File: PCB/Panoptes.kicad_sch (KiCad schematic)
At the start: 104 parts, among them J1 Conn_02x05_Odd_Even, J2 Conn_02x10_Odd_Even, J3 Conn_01x02, J4 Conn_01x03, J5 Conn_01x03, J6 Conn_01x02, J7 Conn_01x02, Q1 MMBT3904, U1 SE555D, U2 ADS7882, U3 L79L05_SOT89, U4 L78L33_SOT89, U5 L78L05_SOT89, U6 OPA2350UA, U7 OPA2350UA, U8 SK0530

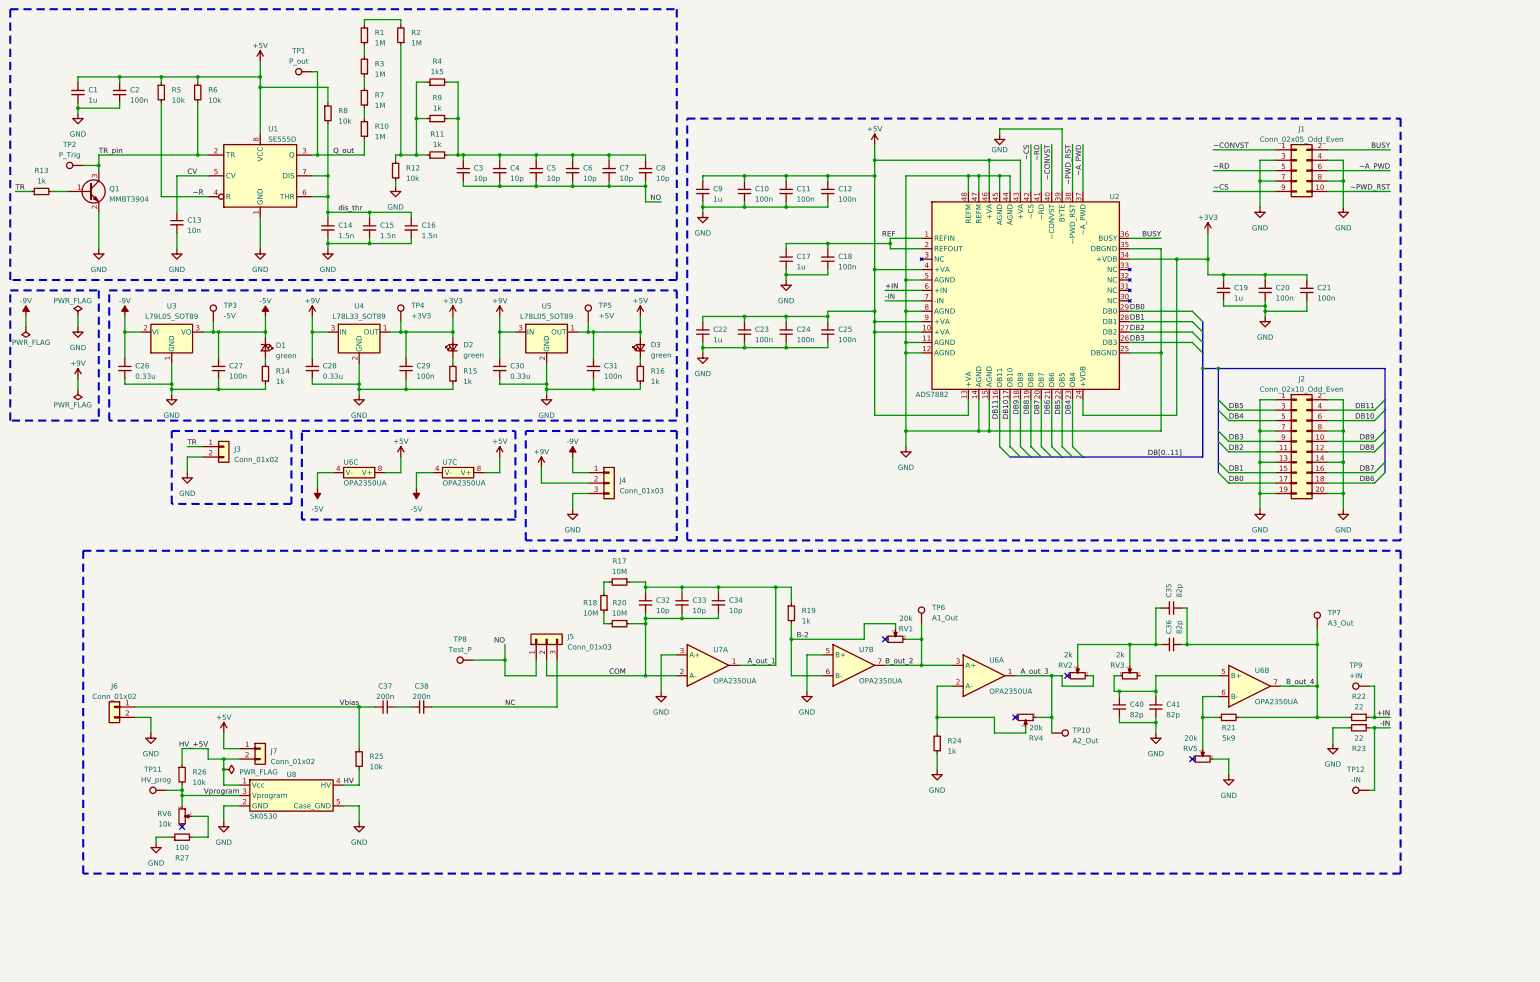
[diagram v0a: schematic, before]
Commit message: V3 completed
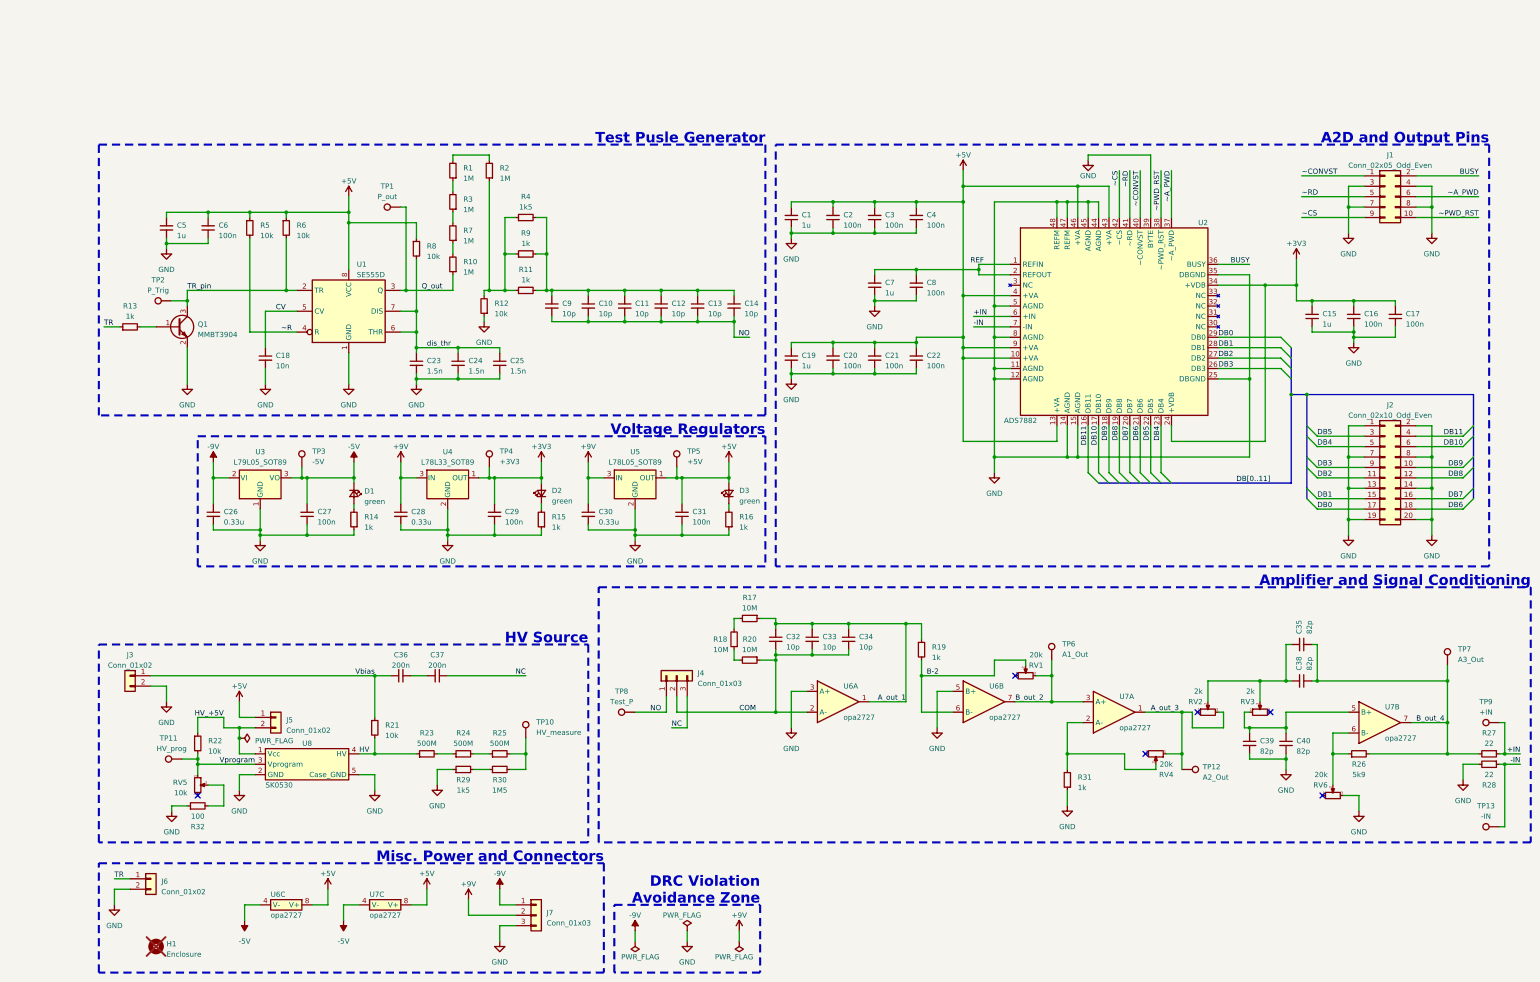
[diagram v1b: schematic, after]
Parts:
- removed U6, U7: OPA2350UA, Package_SO:SOIC-8_3.9x4.9mm_P1.27mm, symbol Panoptes:OPA2350UA
- added H1: Enclosure, n/a, symbol Mechanical:MountingHole
- added R23, R24, R25: 500M, Resistor_THT:R_Axial_DIN0207_L6.3mm_D2.5mm_P7.62mm_Horizontal, symbol Device:R_Small
- added R29: 1k5, Resistor_SMD:R_1206_3216Metric, symbol Device:R_Small
- added R30: 1M5, Resistor_SMD:R_1206_3216Metric, symbol Device:R_Small
- added TP10: HV_measure, TestPoint:TestPoint_Pad_D1.0mm, symbol Connector:TestPoint
- added U6, U7: opa2727, Package_DFN_QFN:DFN-8-1EP_3x3mm_P0.65mm_EP1.55x2.4mm, symbol Panoptes:opa2727
- J1: DK_Detail_Page (none) -> https://www.digikey.com/en/products/detail/sullins-connecto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; DK_PN (none) -> S9202-ND; MPN (none) -> SFH11-PBPC-D05-RA-BK; Manufacturer (none) -> Sullins Connector Solutions
- J2: DK_Detail_Page (none) -> https://www.digikey.com/en/products/detail/sullins-connecto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; DK_PN (none) -> S9205-ND; MPN (none) -> SFH11-PBPC-D10-RA-BK; Manufacturer (none) -> Sullins Connector Solutions
- J4: renamed from J5; DK_Detail_Page (none) -> n/a; DK_PN (none) -> n/a; MPN (none) -> n/a; Manufacturer (none) -> n/a
- J5: renamed from J7; DK_Detail_Page (none) -> n/a; DK_PN (none) -> n/a; MPN (none) -> n/a; Manufacturer (none) -> n/a
- J6: renamed from J3; DK_Detail_Page (none) -> https://www.digikey.com/en/products/detail/sullins-connecto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; DK_PN (none) -> S5438-ND; MPN (none) -> PPTC021LGBN-RC; Manufacturer (none) -> Sullins Connector Solutions
- R1, R10, R2, R3, R7: DK_Detail_Page https://www.digikey.com/en/products/detail/stackpole-electronics-inc/RNCF1206BKE1M00/2027096 -> https://www.digikey.com/en/products/detail/stackpole-electronics-inc/RMCF1206FT1M00/1759703; DK_PN RNCF1206BKE1M00CT-ND -> RMCF1206FT1M00CT-ND; MPN RNCF1206BKE1M00 -> RMCF1206FT1M00
- R11, R13, R14, R15, R16, R19, R9: DK_Detail_Page https://www.digikey.com/en/products/detail/stackpole-electronics-inc/RNCS1206BKE1K00/1800333 -> https://www.digikey.com/en/products/detail/stackpole-electronics-inc/RMCF1206FT1K00/1759616; DK_PN RNCS1206BKE1K00CT-ND -> RMCF1206FT1K00CT-ND; MPN RNCS1206BKE1K00 -> RMCF1206FT1K00
- R12, R5, R6, R8: DK_Detail_Page https://www.digikey.com/en/products/detail/stackpole-electronichttps://www.digikey.com/en/products/detail/stackpole-electronics-inc/RNCS1206BKE10K0/1800330s-inc/RNCS1206BKE10K0/1800330 -> https://www.digikey.com/en/products/detail/stackpole-electronics-inc/RMCF1206FT10K0/1759669; DK_PN RNCS1206BKE10K0CT-ND -> RMCF1206FT10K0CT-ND; MPN RNCS1206BKE10K0 -> RMCF1206FT10K0
- R17, R18, R20: DK_Detail_Page https://www.digikey.com/en/products/detail/vishay-beyschlag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 -> https://www.digikey.com/en/products/detail/stackpole-electr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; DK_PN 749-MCA1206MD1005BP500CT-ND -> RMCF1206FT10M0CT-ND; MPN MCA1206MD1005BP500 -> RMCF1206FT10M0; Manufacturer Vishay Dale -> Stackpole Electronics Inc
- R21: renamed from R25; DK_Detail_Page https://www.digikey.com/en/products/detail/stackpole-electronichttps://www.digikey.com/en/products/detail/stackpole-electronics-inc/RNCS1206BKE10K0/1800330s-inc/RNCS1206BKE10K0/1800330 -> https://www.digikey.com/en/products/detail/stackpole-electronics-inc/RMCF1206FT10K0/1759669; DK_PN RNCS1206BKE10K0CT-ND -> RMCF1206FT10K0CT-ND; MPN RNCS1206BKE10K0 -> RMCF1206FT10K0
- R22: renamed from R26; DK_Detail_Page https://www.digikey.com/en/products/detail/stackpole-electronichttps://www.digikey.com/en/products/detail/stackpole-electronics-inc/RNCS1206BKE10K0/1800330s-inc/RNCS1206BKE10K0/1800330 -> https://www.digikey.com/en/products/detail/stackpole-electronics-inc/RMCF1206FT10K0/1759669; DK_PN RNCS1206BKE10K0CT-ND -> RMCF1206FT10K0CT-ND; MPN RNCS1206BKE10K0 -> RMCF1206FT10K0
- R26: renamed from R21; DK_Detail_Page https://www.digikey.com/en/products/detail/panasonic-electr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 -> https://www.digikey.com/en/products/detail/vishay-dale/CRCW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; DK_PN P5.9KBCCT-ND -> 541-5.90KFCT-ND; MPN ERA-8AEB5901V -> CRCW12065K90FKEA; Manufacturer Panasonic Electronic Components -> Vishay Dale
- R27: renamed from R22; DK_Detail_Page https://www.digikey.com/en/products/detail/stackpole-electronics-inc/RTAN1206BKE22R0/6602201 -> https://www.digikey.com/en/products/detail/stackpole-electronics-inc/RMCF1206FT22R0/1759698; DK_PN RTAN1206BKE22R0CT-ND -> RMCF1206FT22R0CT-ND; MPN RTAN1206BKE22R0 -> RMCF1206FT22R0
- R28: renamed from R23; DK_Detail_Page https://www.digikey.com/en/products/detail/stackpole-electronics-inc/RTAN1206BKE22R0/6602201 -> https://www.digikey.com/en/products/detail/stackpole-electronics-inc/RMCF1206FT22R0/1759698; DK_PN RTAN1206BKE22R0CT-ND -> RMCF1206FT22R0CT-ND; MPN RTAN1206BKE22R0 -> RMCF1206FT22R0
- R31: renamed from R24; DK_Detail_Page https://www.digikey.com/en/products/detail/stackpole-electronics-inc/RNCS1206BKE1K00/1800333 -> https://www.digikey.com/en/products/detail/stackpole-electronics-inc/RMCF1206FT1K00/1759616; DK_PN RNCS1206BKE1K00CT-ND -> RMCF1206FT1K00CT-ND; MPN RNCS1206BKE1K00 -> RMCF1206FT1K00
- R32: renamed from R27; DK_Detail_Page https://www.digikey.com/en/products/detail/yageo/RT1206DRE0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 -> https://www.digikey.com/en/products/detail/stackpole-electr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; DK_PN 311-2954-1-ND -> RMCF1206FG100RCT-ND; MPN RT1206DRE07100RL -> RMCF1206FG100R; Manufacturer YAGEO -> Stackpole Electronics Inc
- R4: DK_Detail_Page https://www.digikey.com/en/products/detail/panasonic-electr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 -> https://www.digikey.com/en/products/detail/stackpole-electr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; DK_PN P1.5KBCCT-ND -> RMCF1206FT1K50CT-ND; MPN ERA-8AEB152V -> RMCF1206FT1K50; Manufacturer Panasonic Electronic Components -> Stackpole Electronics Inc
- TP1, TP2, TP3, TP4, TP5, TP6, TP7, TP8, TP9: footprint TestPoint:TestPoint_Pad_D1.0mm -> Connector_PinHeader_2.54mm:PinHeader_1x01_P2.54mm_Vertical
- TP12: renamed from TP10; footprint TestPoint:TestPoint_Pad_D1.0mm -> Connector_PinHeader_2.54mm:PinHeader_1x01_P2.54mm_Vertical
- TP13: renamed from TP12; footprint TestPoint:TestPoint_Pad_D1.0mm -> Connector_PinHeader_2.54mm:PinHeader_1x01_P2.54mm_Vertical
- renumbered C9 to C1, C4 to C10, C5 to C11, C6 to C12, C7 to C13, C8 to C14, C19 to C15, C20 to C16, C21 to C17, C13 to C18, C22 to C19, C10 to C2, C23 to C20, C24 to C21, C25 to C22, C14 to C23, C15 to C24, C16 to C25, C11 to C3, C37 to C36, C38 to C37, C36 to C38, C40 to C39, C12 to C4, C41 to C40, C1 to C5, C2 to C6, C17 to C7, C18 to C8, C3 to C9, J6 to J3, J4 to J7, RV6 to RV5, RV5 to RV6
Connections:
- net +5V: now also U6.8 (V+), U7.8 (V+)
- net -5V: now also U6.4 (V-), U7.4 (V-)
- net A_out_1: now also U6.1
- net A_out_3: now also U7.1
- net B-2: now also U6.6 (B-)
- net B_out_2: now also U6.7, U7.3 (A+)
- net B_out_4: now also U7.7
- net COM: now also U6.2 (A-)
- net GND: now also R29.1, U6.3 (A+), U6.5 (B+)
- net HV: now also R23.1
- net at C39.1, C40.1, RV3.1: now also U7.5 (B+)
- net at R31.2, RV4.2: now also U7.2 (A-)
- net at R26.1, RV6.2: now also U7.6 (B-)
- new net: R24.2, R25.1
- new net: R25.2, R30.2, TP10.1
- new net: R29.2, R30.1
- new net: R23.2, R24.1
- no-connect marks 5 -> 6
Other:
- note added: "A2D and Output Pins"
- note added: "Amplifier and Signal Conditioning"
- note added: "DRC Violation Avoidance Zone"
- note added: "HV Source"
- note added: "Misc. Power and Connectors"
- note added: "Test Pusle Generator"
- note added: "Voltage Regulators"
- company: (none) -> J. Jackson
- title: (none) -> Panoptes Analog Board Schematic
- moved on the sheet: C1, C10, C11, C12, C13, C14, C15, C16, C17, C18, C19, C2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
